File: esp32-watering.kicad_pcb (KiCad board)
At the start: 2 copper layers, 75 x 55.5 mm, 25 parts, among them J1 5V, J2 12V, J3 Float, J4 Pump, J5 Zone 1, J6 Zone 2, J7 Zone 3, K1 Pump Control, K2 Zone 1, K3 Zone 2, K4 Zone 3, Q1 2N3904, Q2 2N3904, Q3 2N3904, Q4 2N3904, U1 esp32-wemos-d1-mini

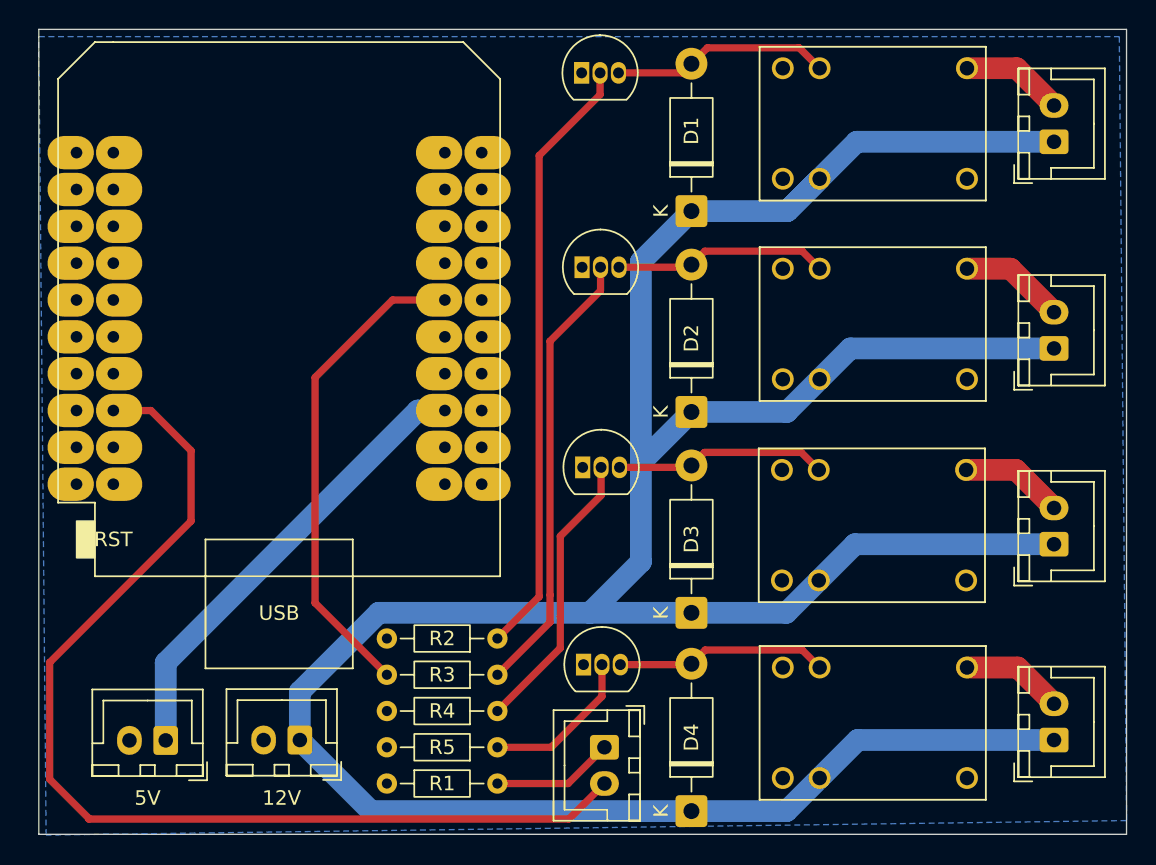
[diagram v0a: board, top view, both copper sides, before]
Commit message: Pre-DRC
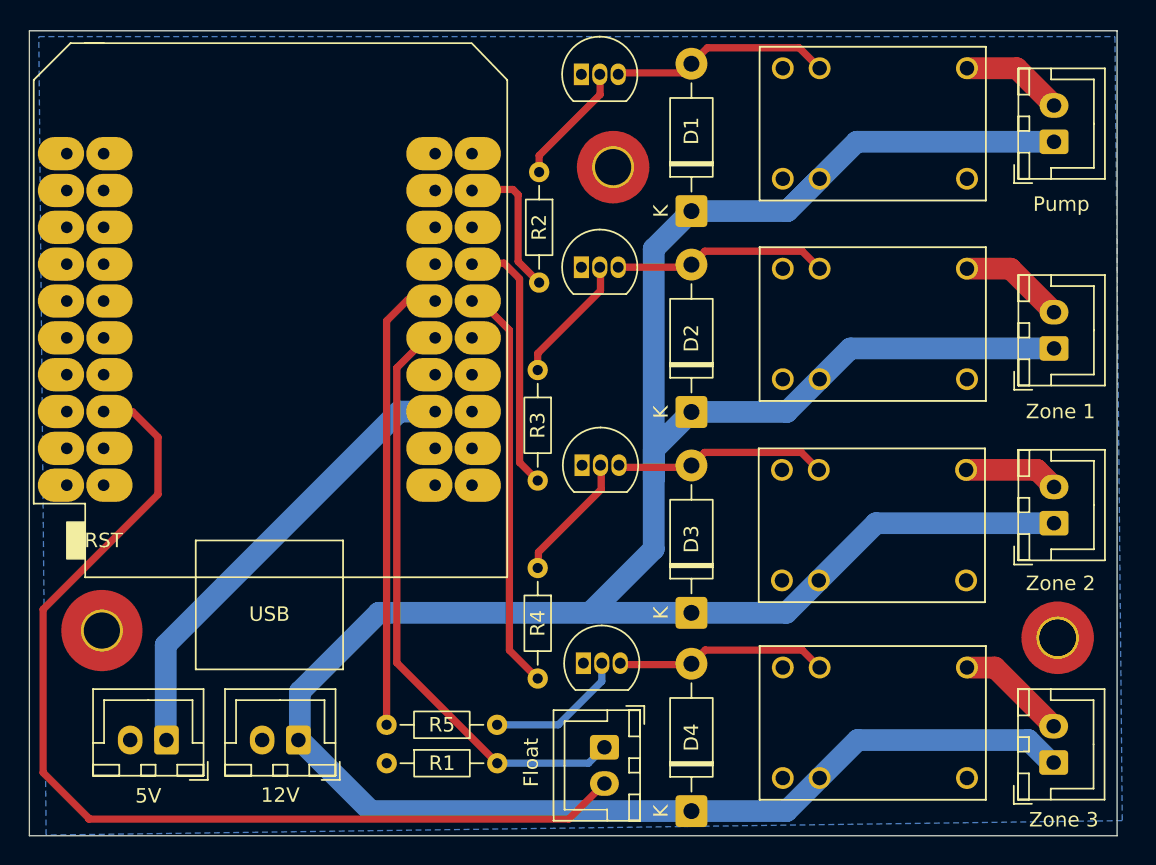
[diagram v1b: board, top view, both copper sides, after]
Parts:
- added ?: , , F.Cu at (126.3, 66.5)
- added ?: , , F.Cu at (192.2, 67.0)
- added REF**: MountingHole_2.5mm_Pad_TopOnly, MountingHole:MountingHole_2.5mm_Pad_TopOnly, F.Cu at (126.3, 66.5)
- added REF**: MountingHole_2.5mm_Pad_TopOnly, MountingHole:MountingHole_2.5mm_Pad_TopOnly, F.Cu at (192.2, 67.0)
- added REF**: MountingHole_2.5mm_Pad_TopOnly, MountingHole:MountingHole_2.5mm_Pad_TopOnly, F.Cu at (161.6, 34.5)
- moved R2 32.3 mm to (156.5, 34.8), turned to -90 degrees
- moved R3 21.2 mm to (156.4, 48.5), turned to -90 degrees
- moved R4 10.2 mm to (156.4, 62.1), turned to -90 degrees
- moved J7 1.55 mm to (192.0, 75.5)
- moved R5 1.55 mm to (153.6, 73.0)
- moved J6 1.45 mm to (192.0, 59.0)
- moved R1 1.40 mm to (146.0, 75.6)
- moved U1 0.67 mm to (137.9, 45.0)
- moved Q3 0.16 mm to (159.5, 55.0)
- moved Q1 0.10 mm to (159.4, 28.1)
- moved Q4 0.10 mm to (159.6, 68.7)
- moved J2 0.10 mm to (139.9, 74.0)
- moved J1 0.06 mm to (130.8, 74.0)
- moved Q2 0.05 mm to (159.4, 41.4)
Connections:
- R2 pad 2: Net-(U1-IO_12/TDI) -> Net-(U1-IO_27)
- R3 pad 2: Net-(U1-IO_17/D3) -> Net-(U1-IO_32)
- R4 pad 2: Net-(U1-IO_32) -> Net-(U1-IO_12/TDI)
- R5 pad 2: Net-(U1-IO_25) -> Net-(U1-IO_17/D3)
- U1 pad 24: Net-(J3-Pin_1) -> Net-(U1-IO_27)
- U1 pad 26: Net-(U1-IO_25) -> unconnected-(U1-IO_25-Pad26)
- U1 pad 31: unconnected-(U1-IO_16/D4-Pad31) -> Net-(J3-Pin_1)
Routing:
- net Net-(Q1-B): track 41.9 -> 8.73 mm
- net Net-(J3-Pin_1): track 8.42 -> 40.9 mm
- net Net-(U1-IO_12/TDI): track 0.00 -> 27.7 mm
- net Net-(Q2-B): track 31.0 -> 9.24 mm
- net Net-(U1-IO_32): track 0.00 -> 17.5 mm
- net Net-(Q3-B): track 19.8 -> 9.24 mm
- net Net-(U1-IO_27): track 0.00 -> 9.32 mm
- net +12V: track 208.1 -> 209.9 mm
- net +3.3V: track 73.6 -> 72.0 mm
- net Net-(U1-IO_17/D3): track 33.7 -> 32.2 mm
- net Net-(Q4-B): track 10.9 -> 9.71 mm
- net Net-(J7-Pin_2): track 7.04 -> 7.65 mm
- net Net-(J6-Pin_2): track 7.15 -> 6.55 mm
